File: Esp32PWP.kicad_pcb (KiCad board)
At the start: 2 copper layers, 24 parts, among them Q1 MMDT2222A, U1 SRV05-4, U2 STUSB4500QTR, U3 STM32L151C8Tx, U4 STM32F030C8Tx, U5 CP2102N-Axx-xQFN28

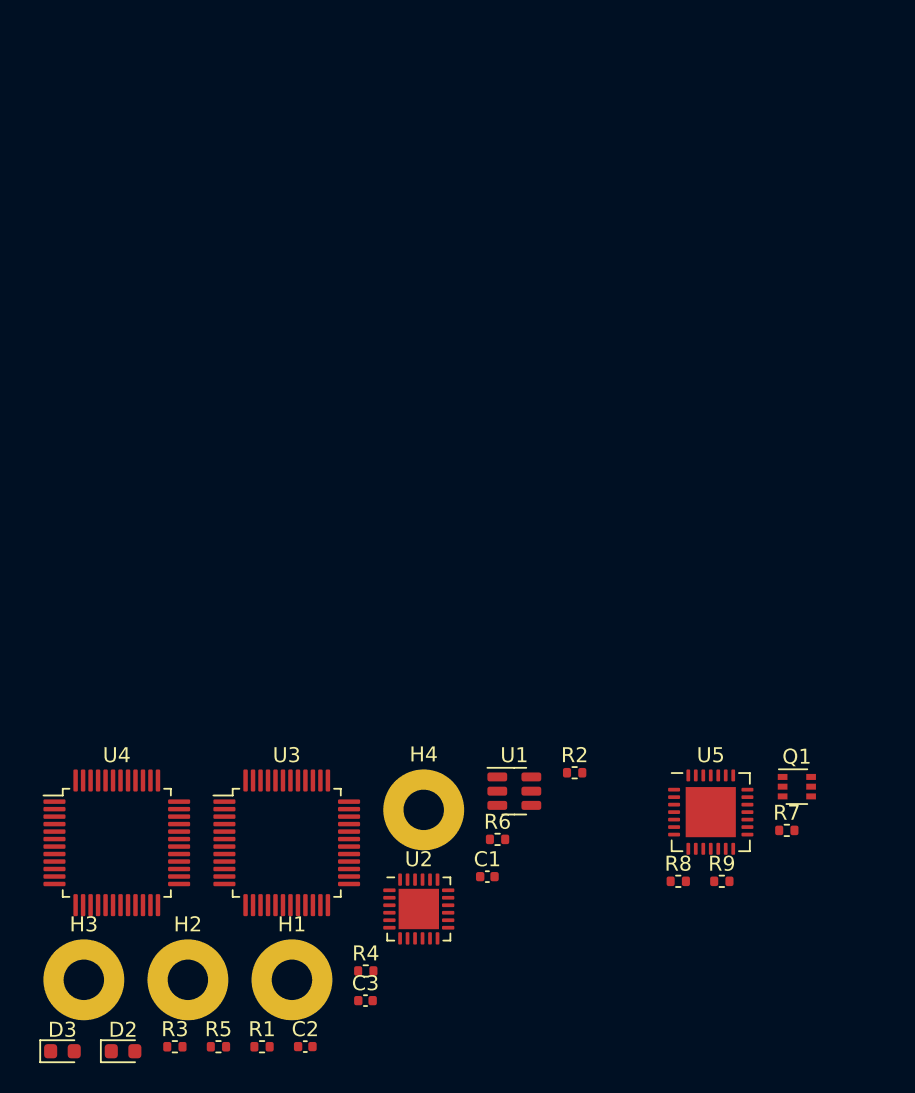
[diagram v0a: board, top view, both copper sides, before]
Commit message: wip
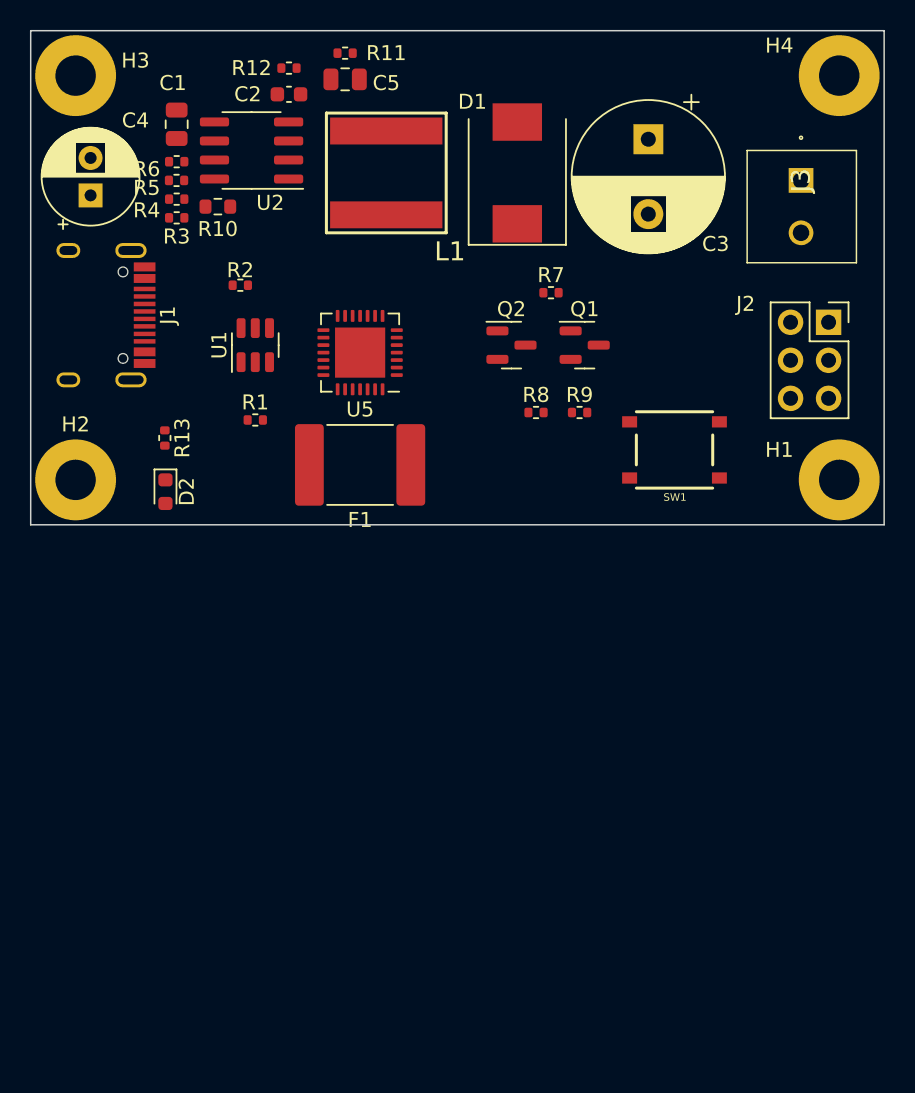
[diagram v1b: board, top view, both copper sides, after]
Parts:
- removed D3: LED_BLUE, LED_SMD:LED_0603_1608Metric
- removed U3: STM32L151C8Tx, Package_QFP:LQFP-48_7x7mm_P0.5mm
- removed U4: STM32F030C8Tx, Package_QFP:LQFP-48_7x7mm_P0.5mm
- added C4: 100u/35V, Capacitor_THT:CP_Radial_D6.3mm_P2.50mm, F.Cu at (116.0, 50.0)
- added C5: 10u/50V, Capacitor_SMD:C_0805_2012Metric, F.Cu at (133.0, 42.2)
- added D1: D_Schottky, Diode_SMD:D_SMC, F.Cu at (144.5, 48.5)
- added F1: 2920L150DR, Fuse:Fuse_2920_7451Metric, F.Cu at (134.0, 68.0)
- added J1: HRO-TYPE-C-31-M-12, Local:HRO-TYPE-C-31-M-12, F.Cu at (111.9, 58.0)
- added J2: Conn_02x03_Odd_Even, Connector_PinSocket_2.54mm:PinSocket_2x03_P2.54mm_Vertical, F.Cu at (165.3, 58.5)
- added J3: Conn_01x02, Local:1985807, F.Cu at (163.4, 49.0)
- added L1: 68uH/1.2A, Local:NR8040T680M, F.Cu at (135.8, 48.5)
- added Q2: MMBT3904, Package_TO_SOT_SMD:SOT-23, F.Cu at (144.1, 60.0)
- added R10: 180R, Resistor_SMD:R_0603_1608Metric, F.Cu at (124.5, 50.8)
- added R11: 20k, Resistor_SMD:R_0402_1005Metric, F.Cu at (133.0, 40.5)
- added R12: 1.2k, Resistor_SMD:R_0402_1005Metric, F.Cu at (129.2, 41.5)
- added R13: 2.7k, Resistor_SMD:R_0402_1005Metric, F.Cu at (121.0, 66.2)
- added SW1: SW_Push, Local:TS-1187A-B-A-B, F.Cu at (155.0, 67.0)
- C1: value 1u/25V -> 10u/50V; footprint Capacitor_SMD:C_0402_1005Metric -> Capacitor_SMD:C_0805_2012Metric
- C2: value 1u/25V -> 680p; footprint Capacitor_SMD:C_0402_1005Metric -> Capacitor_SMD:C_0603_1608Metric
- C3: value 1u/25V -> 330u/35V; footprint Capacitor_SMD:C_0402_1005Metric -> Capacitor_THT:CP_Radial_D10.0mm_P5.00mm
- Q1: value MMDT2222A -> MMBT3904; footprint Package_TO_SOT_SMD:SOT-363_SC-70-6 -> Package_TO_SOT_SMD:SOT-23
- R1: value 10k -> 5.1k
- R2: value 100k -> 5.1k
- R3: value 470R -> 1R
- R4: value 1k -> 1R
- R5: value 100k -> 1R
- R6: value 200R -> 1R
- U2: value STUSB4500QTR -> MC34063AD; footprint Package_DFN_QFN:QFN-24-1EP_4x4mm_P0.5mm_EP2.7x2.7mm -> Package_SO:SOIC-8_3.9x4.9mm_P1.27mm
- moved C2 63.6 mm to (129.2, 43.2), turned to 180 degrees
- moved C3 60.6 mm to (153.2, 46.2), turned to -90 degrees
- moved H3 60.4 mm to (115.0, 42.0)
- moved R5 57.9 mm to (121.7, 49.0), turned to 180 degrees
- moved H4 56.3 mm to (166.0, 42.0)
- moved R3 55.4 mm to (121.8, 51.5), turned to 180 degrees
- moved C1 54.4 mm to (121.8, 45.2), turned to 90 degrees
- moved R4 53.1 mm to (121.8, 50.2), turned to 180 degrees
- moved U2 51.9 mm to (126.8, 47.0), turned to 180 degrees
- moved R6 50.1 mm to (121.8, 47.8), turned to 180 degrees
- moved H1 49.5 mm to (166.0, 69.0)
- moved R1 41.9 mm to (127.0, 65.0)
- moved R2 39.5 mm to (126.0, 56.0), turned to 180 degrees
- moved R7 39.2 mm to (146.8, 56.5)
- moved U5 38.6 mm to (134.0, 60.5), turned to 180 degrees
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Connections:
- C1 pad 1: Net-(C1-Pad1) -> VBUS
- C3 pad 1: Net-(C3-Pad1) -> +24V
- D2 pad 1: unconnected-(D2-Pad1) -> GND
- D2 pad 2: unconnected-(D2-Pad2) -> Net-(D2-Pad2)
- Q1 pad 1: /USB2serial/RTS -> Net-(R7-Pad1)
- Q1 pad 2: Net-(Q1-Pad2) -> /USB2serial/RTS
- Q1 pad 3: /USB2serial/IO0 -> /USB2serial/CHIP_PU
- R1 pad 1: Net-(R1-Pad1) -> /CC2
- R2 pad 1: Net-(R2-Pad1) -> /CC1
- R3 pad 1: VBUS -> Net-(L1-Pad1)
- R3 pad 2: Net-(C1-Pad1) -> VBUS
- R4 pad 1: Net-(C1-Pad1) -> Net-(L1-Pad1)
- R4 pad 2: Net-(R4-Pad2) -> VBUS
- R5 pad 1: Net-(R5-Pad1) -> Net-(L1-Pad1)
- R5 pad 2: GND -> VBUS
- R6 pad 1: VBUS -> Net-(L1-Pad1)
- R6 pad 2: Net-(R6-Pad2) -> VBUS
- R7 pad 1: Net-(Q1-Pad2) -> Net-(R7-Pad1)
- R8 pad 1: Net-(Q1-Pad5) -> Net-(R8-Pad1)
- U1 pad 5: +5V -> VBUS
- U2 pad 1: /CC1 -> Net-(D1-Pad2)
- U2 pad 2: /CC1 -> GND
- U2 pad 3: unconnected-(U2-Pad3) -> Net-(C2-Pad1)
- U2 pad 4: /CC2 -> GND
- U2 pad 5: /CC2 -> Net-(R11-Pad2)
- U2 pad 6: Net-(R1-Pad1) -> VBUS
- U2 pad 7: GND -> Net-(L1-Pad1)
- U2 pad 8: GND -> Net-(R10-Pad2)
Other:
- board outline added: 57 x 33 mm
